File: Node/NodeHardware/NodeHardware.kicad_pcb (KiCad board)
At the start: 2 copper layers, 149 parts, among them J1 USB_C_Receptacle_16P, Q1 AO3401A, Q2 AO3401A, Q4 2N7002, Q5 2N7002, U3 CH340C, U5 MCP73831-2-OT, U8 UCC27511ADBV

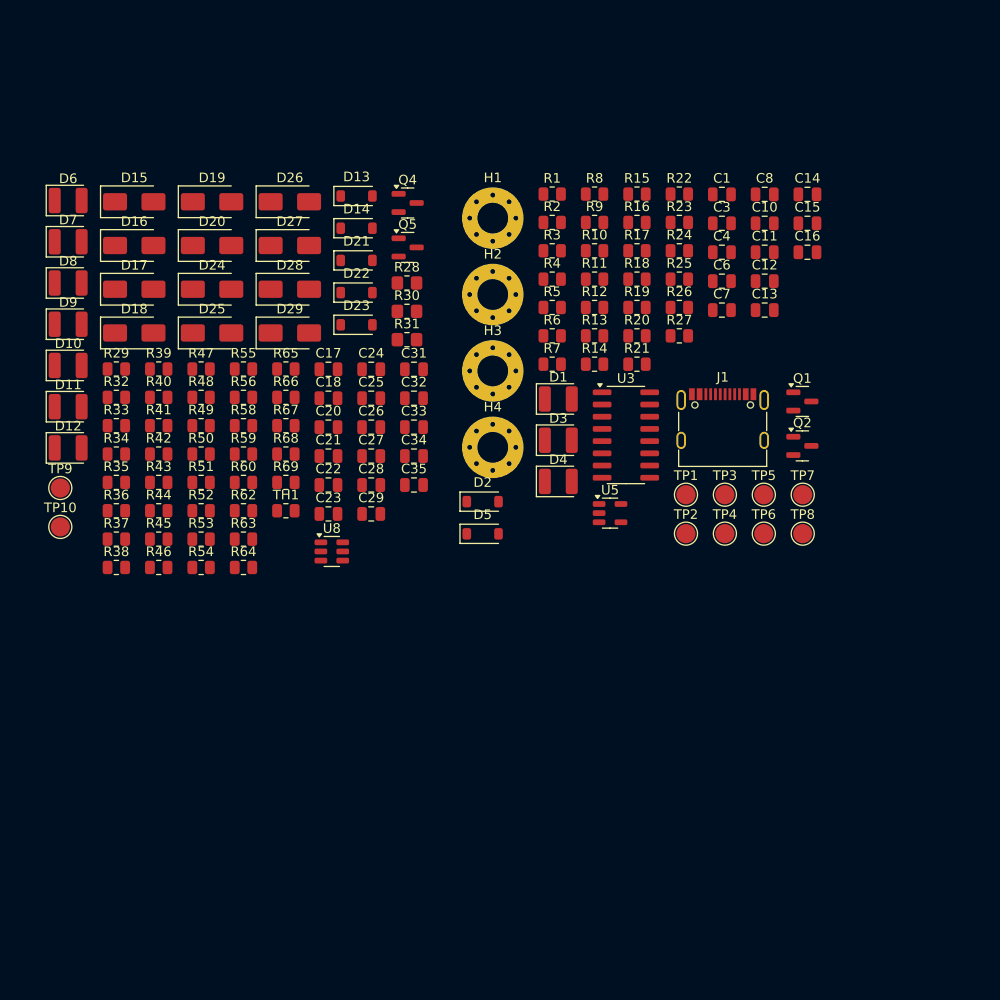
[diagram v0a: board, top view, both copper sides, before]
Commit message: Continue schm update, slow progress
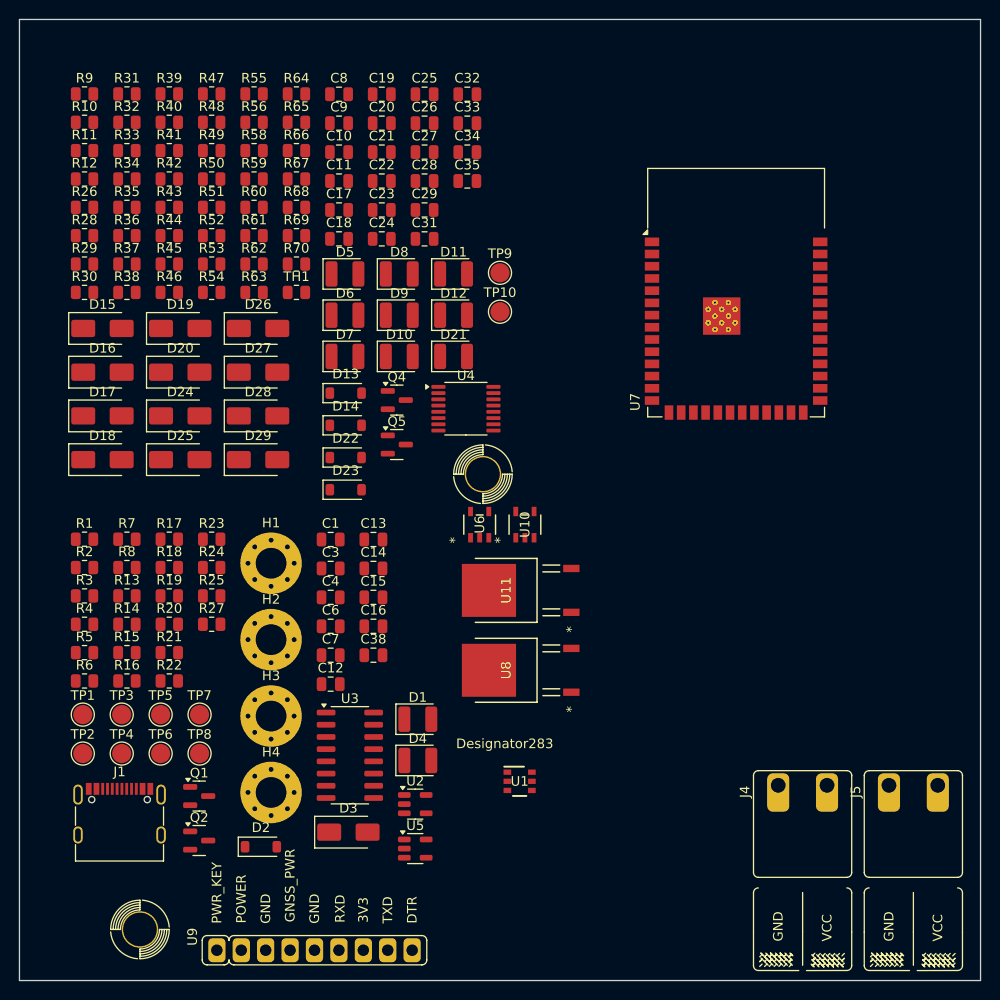
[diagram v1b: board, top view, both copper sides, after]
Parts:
- added C19: 100n, Capacitor_SMD:C_0805_2012Metric, F.Cu at (137.7, 57.8)
- added C38: 10u, Capacitor_SMD:C_0805_2012Metric, F.Cu at (136.8, 116.2)
- added C9: 100n, Capacitor_SMD:C_0805_2012Metric, F.Cu at (133.2, 60.8)
- added J4: PWR_IN, fflori4nComponents:TerminalBlockRemovablex2_Silk, F.Cu at (181.5, 128.2)
- added J5: BATT, fflori4nComponents:TerminalBlockRemovablex2_Silk, F.Cu at (193.0, 128.2)
- added R61: ???, Resistor_SMD:R_0805_2012Metric, F.Cu at (124.4, 72.5)
- added R70: ???, Resistor_SMD:R_0805_2012Metric, F.Cu at (128.8, 75.5)
- added U1: TPS565201DDCR, TPS565201DDCR:TPS565201DDCR_L, F.Cu at (152.0, 129.3)
- added U10: UCC27517DBVR, UCC27517DBVR:UCC27517DBVR_DBV5_TEX, F.Cu at (152.6, 102.6)
- added U11: IRLR024NTRPBF, IRLR024NTRPBF:IRLR024NTRPBF_PG-TO252-3_INF, F.Cu at (150.6, 109.4)
- added U2: SPX3819M5-L-3-3, Package_TO_SOT_SMD:SOT-23-5, F.Cu at (141.2, 131.6)
- added U4: ADS1220xPW, Package_SO:TSSOP-16_4.4x5mm_P0.65mm, F.Cu at (146.5, 90.5)
- added U6: UCC27517DBVR, UCC27517DBVR:UCC27517DBVR_DBV5_TEX, F.Cu at (147.9, 102.6)
- added U7: ESP32-S3-WROOM-1, RF_Module:ESP32-S3-WROOM-1, F.Cu at (174.6, 78.4)
- added U9: SIM7000G_DEVBoard, fflori4nComponents:sim7000G_dev_board_rev3, F.Cu at (120.5, 146.8)
- C10: value 10u -> 100n
- C11: value 1u -> 100n
- D21: value 3V6 -> YELLOW; footprint Diode_SMD:D_SOD-123 -> LED_SMD:LED_1210_3225Metric
- D3: value LED -> SS14; footprint LED_SMD:LED_1210_3225Metric -> Diode_SMD:D_SMA
- D5: value 5V1 -> YELLOW; footprint Diode_SMD:D_SOD-123 -> LED_SMD:LED_1210_3225Metric
- R10: value ??? -> 47k
- R11: value INF -> 47k
- R12: value 4k7 -> 47k
- R15: value 10k -> 0R
- R26: value 47k -> 10k
- R28: value 10K -> 10k; footprint Resistor_SMD:R_0805_2012Metric_Pad1.20x1.40mm_HandSolder -> Resistor_SMD:R_0805_2012Metric
- R30, R31: value 10K -> 47k; footprint Resistor_SMD:R_0805_2012Metric_Pad1.20x1.40mm_HandSolder -> Resistor_SMD:R_0805_2012Metric
- R33, R34, R35, R36, R38, R39: value 2k2 -> 10k
- R37: value 2k2 -> 10kk
- R48, R49, R52, R56: value 220k -> 470R
- R9: value 10k -> 47k
- TP7: value 3V3_TP -> 3V3_Bypass_TP
- TP8: value 3V3_LP_TP -> 3V3_TP
- U8: value UCC27511ADBV -> IRLR024NTRPBF; footprint Package_TO_SOT_SMD:SOT-23-6 -> IRLR024NTRPBF:IRLR024NTRPBF_PG-TO252-3_INF
- moved Q1 75.0 mm to (118.7, 130.8)
- moved Q2 75.0 mm to (118.7, 135.4)
- moved J1 75.0 mm to (110.4, 133.8)
- moved R22 73.4 mm to (115.6, 118.8)
- moved R15 71.4 mm to (111.2, 115.9)
- moved R16 71.4 mm to (111.2, 118.8)
- moved TP3 66.8 mm to (110.6, 122.3)
- moved TP4 66.8 mm to (110.6, 126.4)
- moved TP7 66.8 mm to (118.7, 122.3)
- moved TP8 66.8 mm to (118.7, 126.4)
- moved TP1 66.8 mm to (106.6, 122.3)
- moved TP2 66.8 mm to (106.6, 126.4)
- moved TP5 66.8 mm to (114.7, 122.3)
- moved TP6 66.8 mm to (114.7, 126.4)
- moved R26 62.8 mm to (106.8, 69.5)
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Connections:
- net /MCU_And_Peripherals/UART_RX_LED_K renamed /MCU_And_Peripherals/UART0_RX_LED_K
- net /MCU_And_Peripherals/UART_TX_LED_K renamed /MCU_And_Peripherals/UART0_TX_LED_K
- net 5V_REG_EN renamed Net-(U1-EN)
- net UART_UC_RX renamed UART0_UC_RX
- net UART_UC_TX renamed UART0_UC_TX
- C10 pad 1: +3V3 -> 5V_SENSE
- C11 pad 1: +3V3 -> PWR_SENSE
- C14 pad 1: +3V3_LP -> +3V3
- C23 pad 1: BATT_SENSE -> BATT_N
- C23 pad 2: BATT_N -> +3V3
- C8 pad 1: /3V3_REG_SW -> BATT_SENSE
- C8 pad 2: Net-(U2-VBST) -> BATT_N
- D21 pad 1: /MCU_And_Peripherals/AIN_1 -> /MCU_And_Peripherals/UART1_TX_LED_K
- D21 pad 2: BATT_N -> +3V3
- D3 pad 1: /3V3_REG_LED_K -> +BATT
- D3 pad 2: +3V3 -> BATT_P
- D5 pad 1: +BATT -> /MCU_And_Peripherals/UART1_RX_LED_K
- D5 pad 2: /BATT_IN_ZENER -> +3V3
- Q2 pad 1: /BATT_IN_ZENER -> BATT_N
- R10 pad 1: +3V3 -> BATT_SENSE
- R10 pad 2: /3V3_REG_VFB -> BATT_N
- R11 pad 1: BATT_N -> +3V3
- R11 pad 2: 3V3_REG_EN -> 3V3_SENSE
- R12 pad 1: /3V3_REG_LED_K -> 3V3_SENSE
- R15 pad 1: /3V3_REG_VFB -> +5V
- R15 pad 2: BATT_N -> /3V3_LP_REG_IN
- R17 pad 1: /net_lable -> /CH340_TX
- R19 pad 1: /net_lable -> /CH340_RX
- R26 pad 1: /BATT_IN_ZENER -> /MCU_And_Peripherals/UART1_RX_LED_K
- R26 pad 2: BATT_N -> UART1_UC_RX
- R28 pad 1: /MCU_And_Peripherals/GSM_PWR_KEY -> /MCU_And_Peripherals/UART1_TX_LED_K
- R28 pad 2: +5V -> UART1_UC_TX
- R30 pad 1: unconnected-(R30-Pad1) -> +5V
- R30 pad 2: unconnected-(R30-Pad2) -> 5V_SENSE
- R31 pad 1: unconnected-(R31-Pad1) -> 5V_SENSE
- R31 pad 2: unconnected-(R31-Pad2) -> BATT_N
- R45 pad 1: +BATT -> V_IN
- R45 pad 2: BATT_SENSE -> PWR_SENSE
- R47 pad 1: BATT_SENSE -> PWR_SENSE
- R8 pad 1: +5V -> Net-(U2-EN)
- R8 pad 2: /3V3_REG_IN -> /3V3_LP_REG_IN
- R9 pad 1: /3V3_REG_IN -> +BATT
- R9 pad 2: 3V3_REG_EN -> BATT_SENSE
- TP7 pad 1: +3V3 -> Net-(U2-BP)
- TP8 pad 1: +3V3_LP -> +3V3
- U3 pad 2: /net_lable -> /CH340_TX
- U3 pad 3: /net_lable -> /CH340_RX
- U8 pad 1: unconnected-(U8-V_{DD}-Pad1) -> Net-(U8-G)
- U8 pad 2: unconnected-(U8-OUTH-Pad2) -> DIG_OUT_01
- U8 pad 3: unconnected-(U8-OUTL-Pad3) -> BATT_N
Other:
- board outline added: 100 x 100 mm
